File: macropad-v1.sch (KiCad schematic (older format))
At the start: 24 parts, among them SW1 SW_Push, U1 ATmega32U4-AU, Y1 16MHz

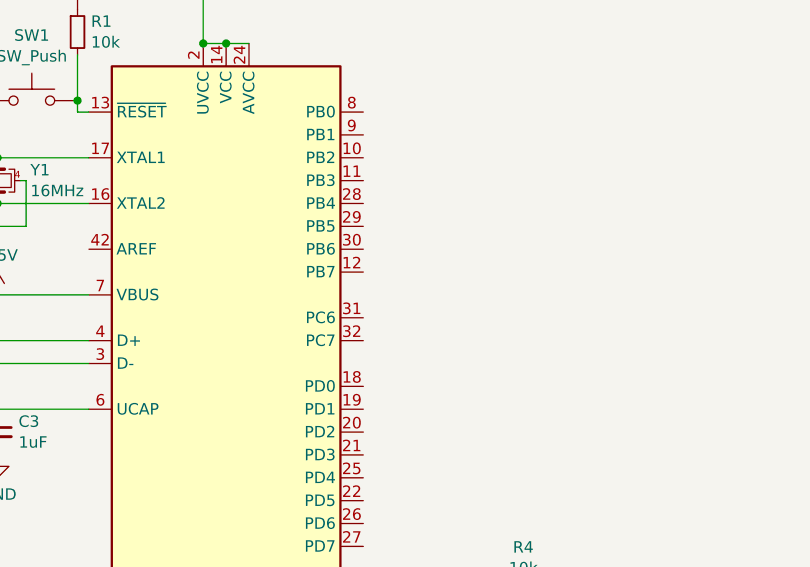
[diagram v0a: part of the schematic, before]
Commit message: pcb routes
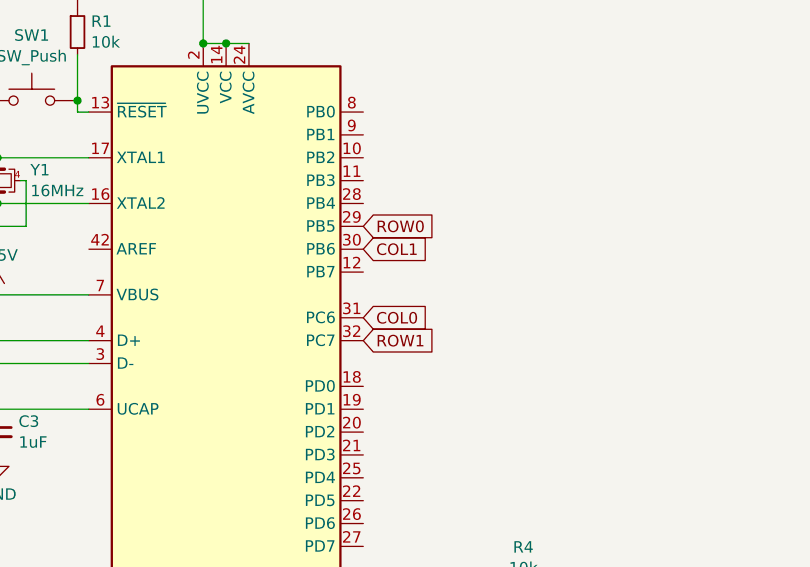
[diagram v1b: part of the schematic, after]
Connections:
- net COL0: now also U1.31 (PC6)
- net COL1: now also U1.30 (PB6)
- net ROW0: now also U1.29 (PB5)
- net ROW1: now also U1.32 (PC7)
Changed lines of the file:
@@
 Text GLabel 7225 4600 0    50   Input ~ 0
 ROW1
+Text GLabel 4900 3325 2    50   Input ~ 0
+COL1
+Text GLabel 4900 3225 2    50   Input ~ 0
+ROW0
+Text GLabel 4900 3625 2    50   Input ~ 0
+COL0
+Text GLabel 4900 3725 2    50   Input ~ 0
+ROW1
 $EndSCHEMATC
